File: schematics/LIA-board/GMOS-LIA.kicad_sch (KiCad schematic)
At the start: 0 parts

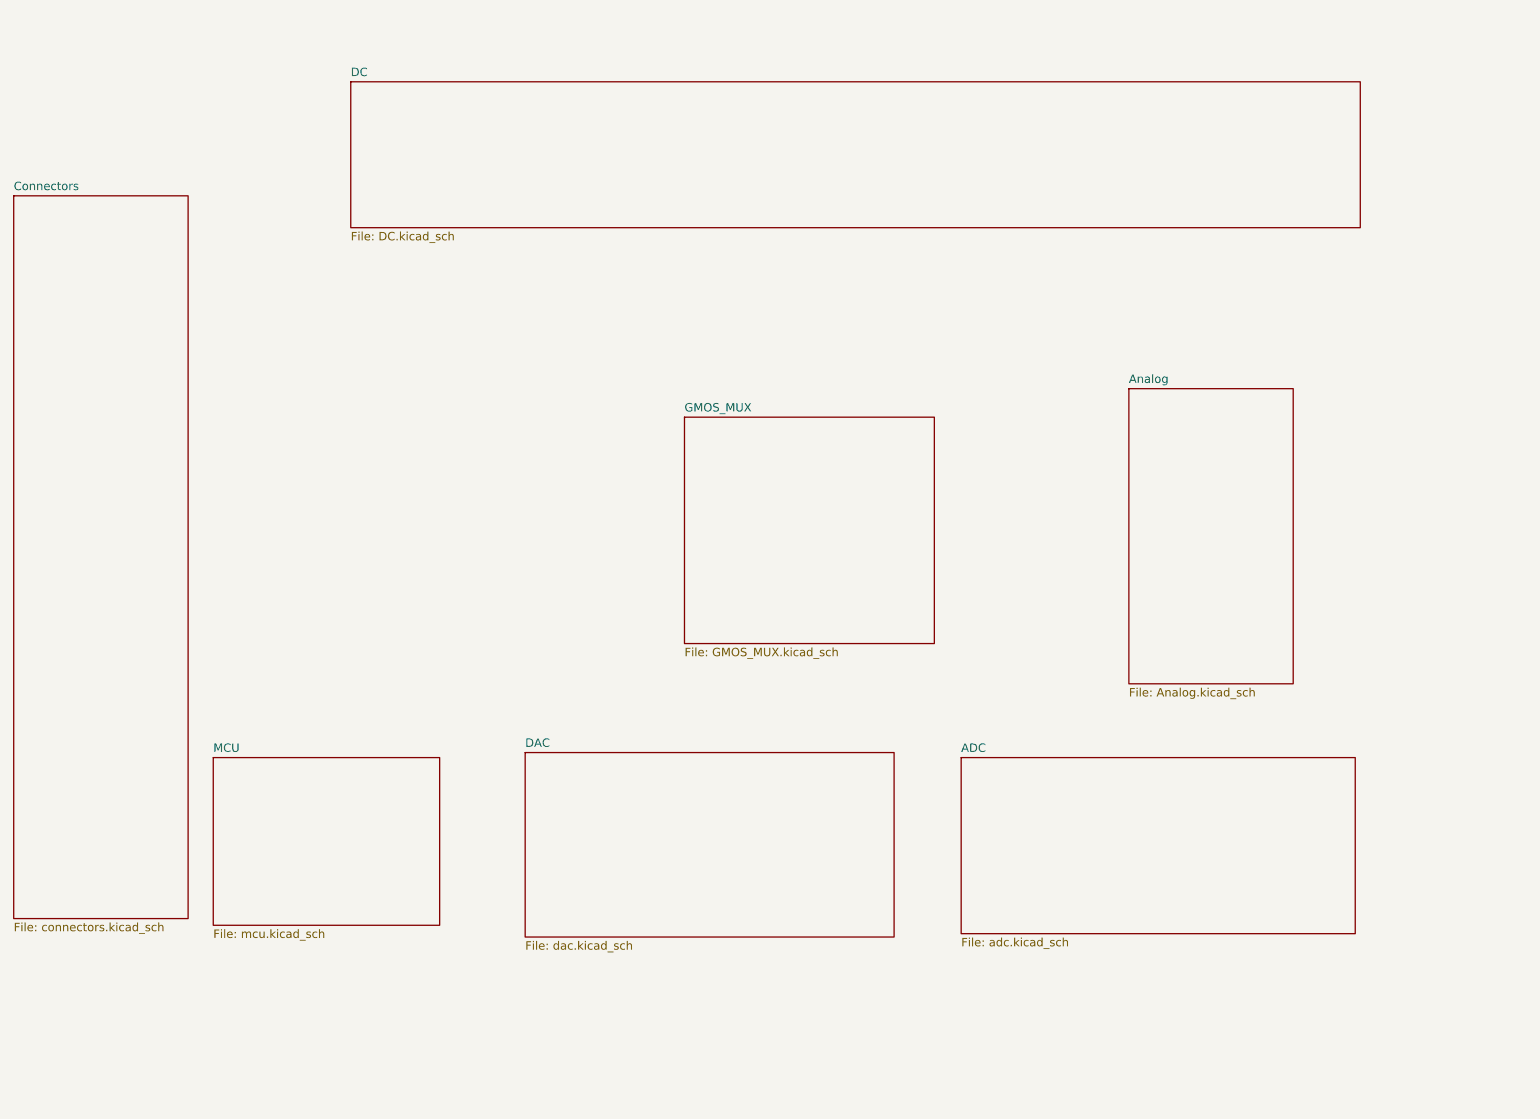
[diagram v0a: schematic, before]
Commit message: commit before changing LIA
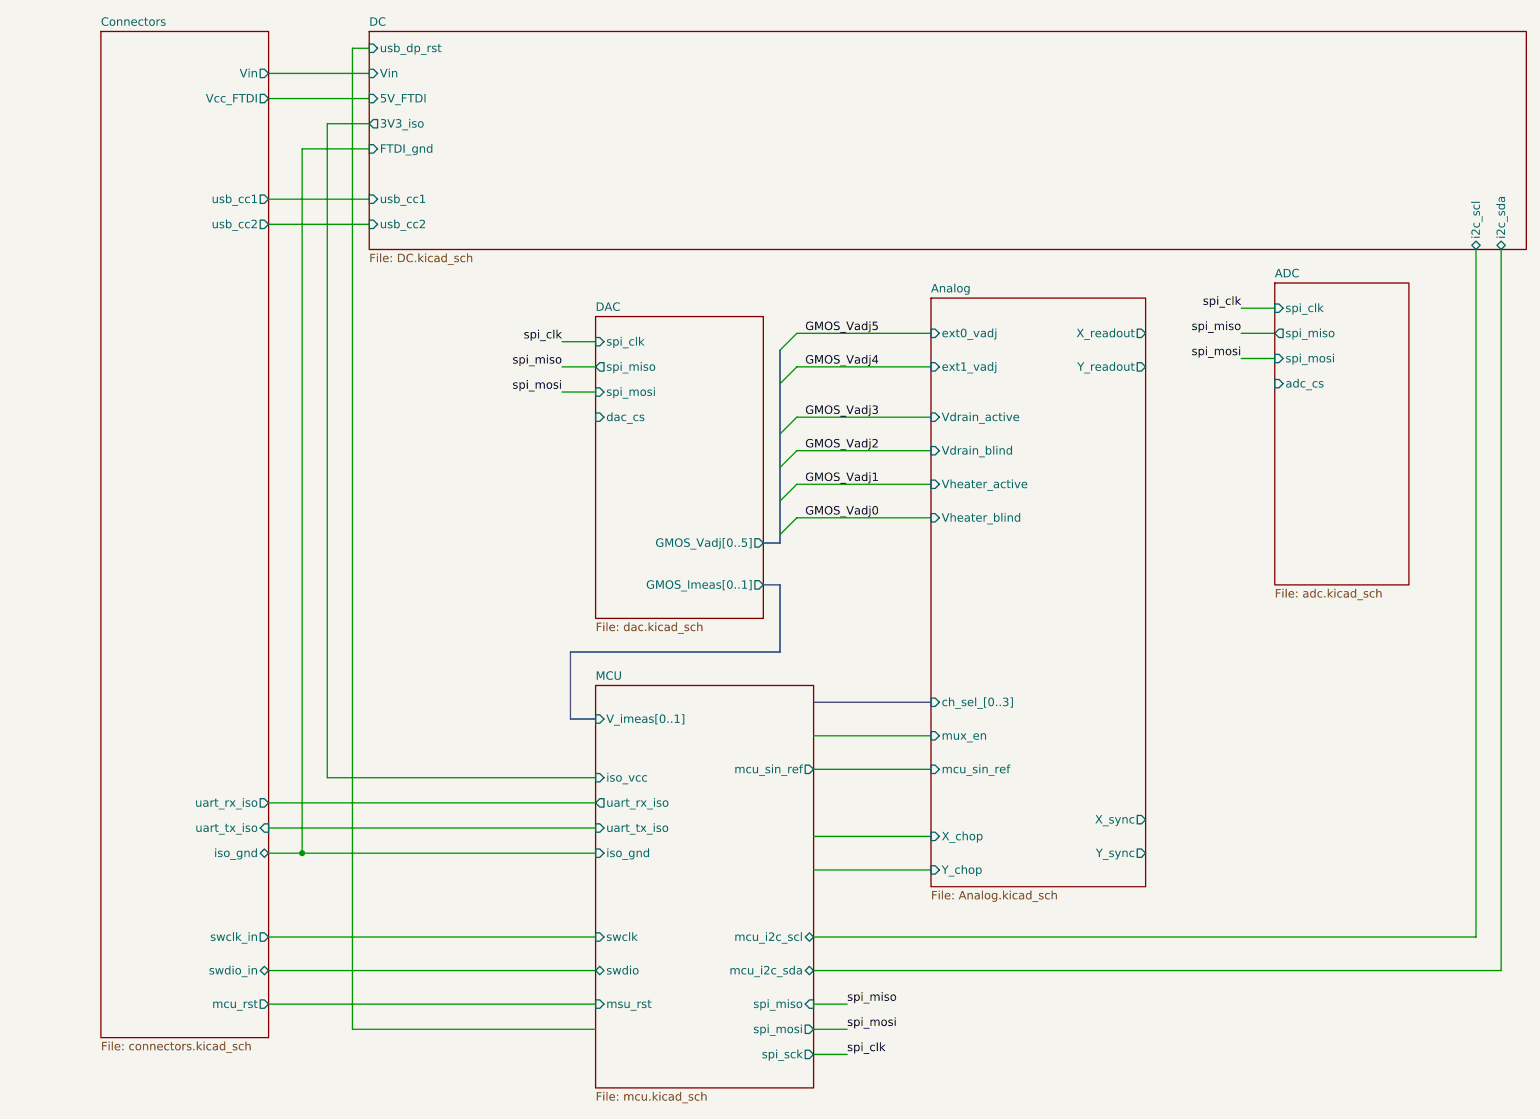
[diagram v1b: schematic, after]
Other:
- removed sheet GMOS_MUX
- sheet ADC ports: added adc_cs, spi_clk, spi_miso, spi_mosi; removed none
- sheet Analog ports: added Vdrain_active, Vdrain_blind, Vheater_active, Vheater_blind, X_chop, X_readout, X_sync, Y_chop, Y_readout, Y_sync, ch_sel_[0..3], ext0_vadj, ext1_vadj, mcu_sin_ref, mux_en; removed none
- sheet Connectors ports: added Vcc_FTDI, Vin, iso_gnd, mcu_rst, swclk_in, swdio_in, uart_rx_iso, uart_tx_iso, usb_cc1, usb_cc2; removed none
- sheet DAC ports: added GMOS_Imeas[0..1], GMOS_Vadj[0..5], dac_cs, spi_clk, spi_miso, spi_mosi; removed none
- sheet DC ports: added 3V3_iso, 5V_FTDI, FTDI_gnd, Vin, i2c_scl, i2c_sda, usb_cc1, usb_cc2, usb_dp_rst; removed none
- sheet MCU ports: added V_imeas[0..1], iso_gnd, iso_vcc, mcu_i2c_scl, mcu_i2c_sda, mcu_sin_ref, msu_rst, spi_miso, spi_mosi, spi_sck, swclk, swdio, uart_rx_iso, uart_tx_iso; removed none
